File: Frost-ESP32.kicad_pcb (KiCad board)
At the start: 4 copper layers, 50 x 50 mm, 31 parts, among them J1 Micro_SD_Card, J2 CAN, J3 USB_C_Receptacle_USB2.0, J4 Conn_01x10, SW1 SW_Push, U1 ESP32-C3-WROOM-02, U2 AP2112K-3.3, U3 TJA1051T-3

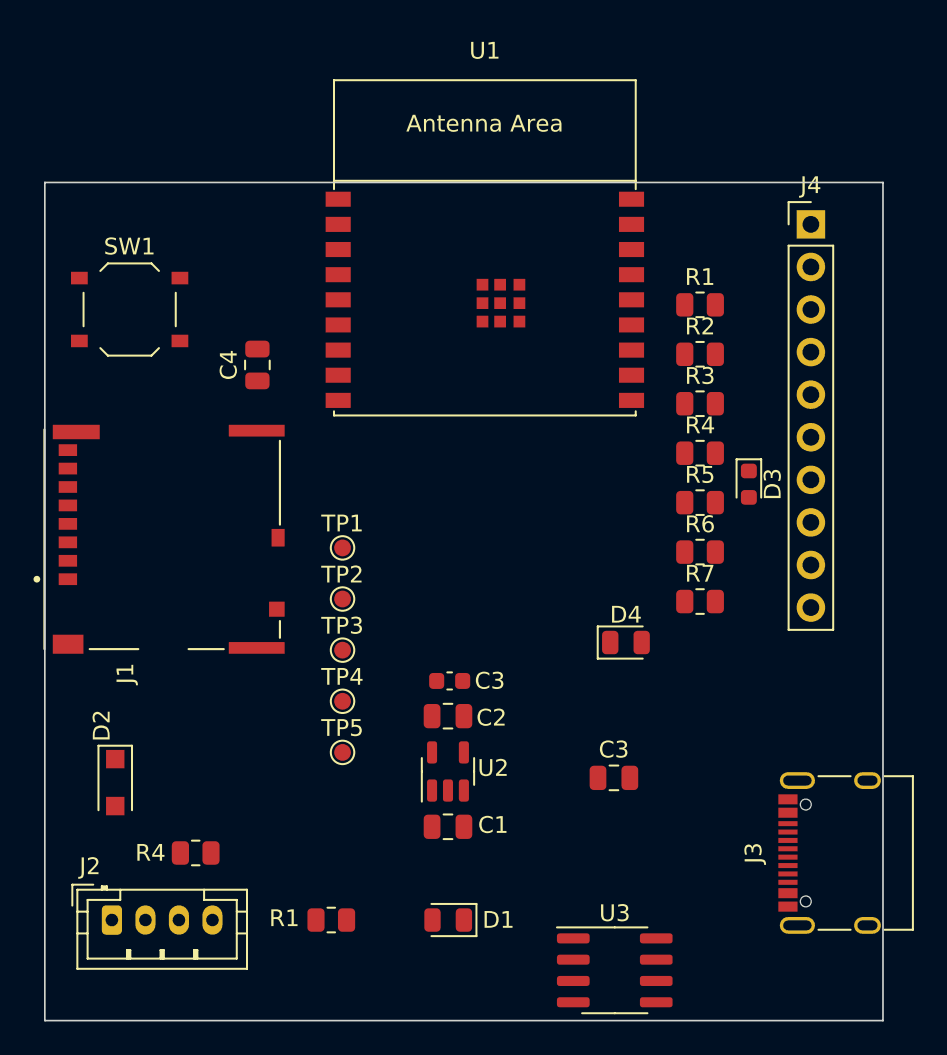
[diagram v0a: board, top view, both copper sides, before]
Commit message: After ordering v0.1
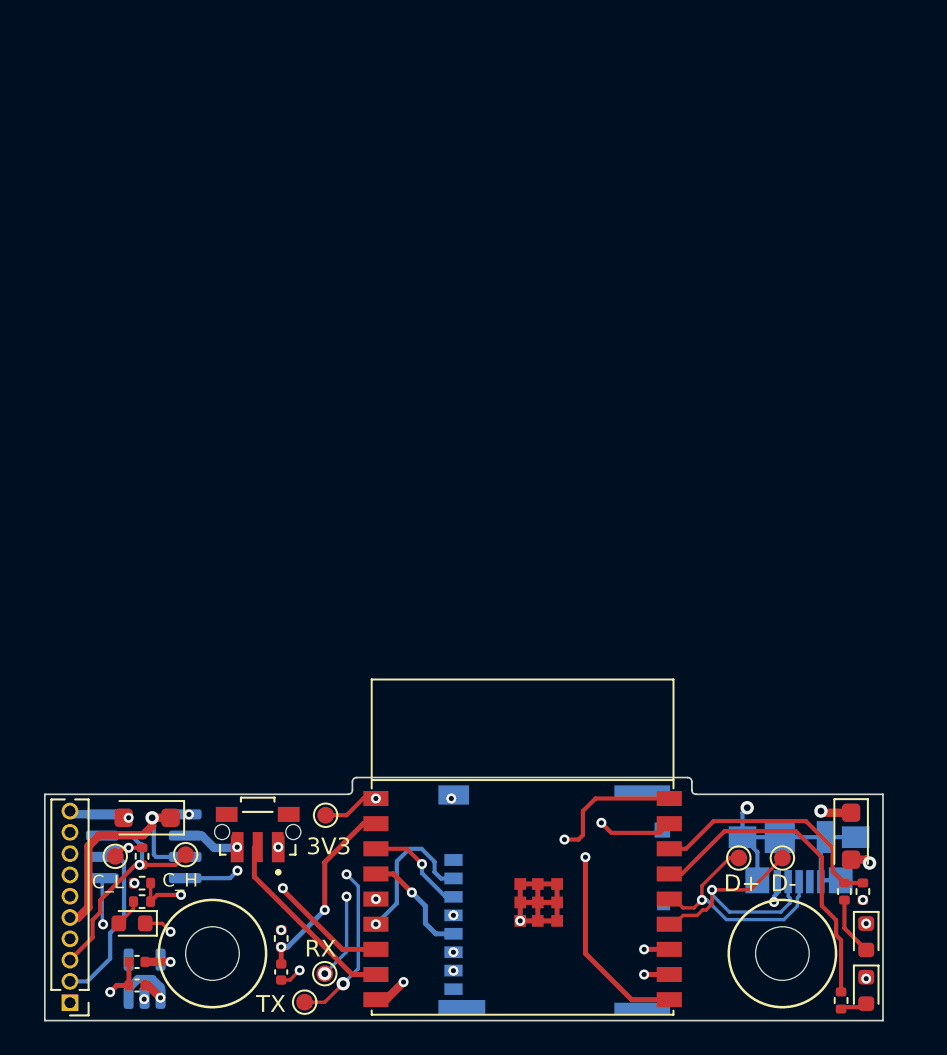
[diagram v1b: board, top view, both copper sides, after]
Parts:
- removed the C3 at (118.2, 90.7)
- removed the C3 at (128.0, 96.5)
- removed C4: 1u, Capacitor_SMD:C_0805_2012Metric
- removed J4: Conn_01x10, Connector_PinHeader_2.54mm:PinHeader_1x10_P2.54mm_Vertical
- removed the R1 at (133.1, 68.3)
- removed the R1 at (111.1, 105.0)
- removed the R4 at (133.1, 77.2)
- removed the R4 at (103.0, 101.0)
- removed SW1: SW_Push, Button_Switch_SMD:SW_Push_1P1T_XKB_TS-1187A
- added C3: 1uF/25V, Capacitor_SMD:C_0402_1005Metric, F.Cu at (108.1, 108.1)
- added D5: 100V/3A, Diode_SMD:D_SOD-123F, F.Cu at (142.1, 100.0)
- added H1: MountingHole, MountingHole:MountingHole_3.2mm_M3, F.Cu at (104.0, 107.0)
- added H2: MountingHole, MountingHole:MountingHole_3.2mm_M3, F.Cu at (138.0, 107.0)
- added R1: 1k, Resistor_SMD:R_0402_1005Metric, F.Cu at (141.7, 103.3)
- added R4: 220, Resistor_SMD:R_0402_1005Metric, F.Cu at (99.8, 101.2)
- added S1: TL3340AF160QG, Fair:SW_TL3340AF160QG, F.Cu at (106.7, 99.8)
- added TP6: TestPoint, TestPoint:TestPoint_Pad_D1.0mm, F.Cu at (110.7, 108.2)
- added TP7: TestPoint, TestPoint:TestPoint_Pad_D1.0mm, F.Cu at (109.5, 109.9)
- C1, C2: value 10uF -> 10uF/6.3V; footprint Capacitor_SMD:C_0805_2012Metric -> Capacitor_SMD:C_0402_1005Metric
- D1: value RED -> Red; footprint LED_SMD:LED_0805_2012Metric -> LED_SMD:LED_0603_1608Metric
- D3: value BLUE -> Blue
- D4: value RED -> Emerald; footprint LED_SMD:LED_0805_2012Metric -> LED_SMD:LED_0603_1608Metric
- J1: footprint espressif:MOLEX_503398-1892 -> Fair:MOLEX_503398-1892; moved to B.Cu
- J2: footprint Connector_JST:JST_PH_B4B-PH-K_1x04_P2.00mm_Vertical -> Connector_PinHeader_1.27mm:PinHeader_1x10_P1.27mm_Vertical
- J3: value USB_C_Receptacle_USB2.0 -> USB__B_Micro_Horizontal; footprint Connector_USB:USB_C_Receptacle_XKB_U262-16XN-4BVC11 -> Connector_USB:USB_Micro-B_Molex_47346-0001; moved to B.Cu
- R2: value R_0805_10k -> 10k; footprint Resistor_SMD:R_0805_2012Metric -> Resistor_SMD:R_0402_1005Metric
- R3, R5, R6, R7: footprint Resistor_SMD:R_0805_2012Metric -> Resistor_SMD:R_0402_1005Metric
- U2, U3: moved to B.Cu
- moved R2 42.9 mm to (108.1, 106.1), turned to 90 degrees
- moved R6 38.7 mm to (99.8, 102.8), turned to 180 degrees
- moved R7 37.8 mm to (99.8, 103.9), turned to 180 degrees
- moved U1 35.8 mm to (122.5, 103.7)
- moved J1 31.5 mm to (124.0, 103.8), turned to -90 degrees
- moved D3 31.0 mm to (143.0, 109.2)
- moved R5 30.9 mm to (141.5, 109.8), turned to 90 degrees
- moved R3 30.7 mm to (142.8, 103.3), turned to 90 degrees
- moved TP2 30.5 mm to (138.0, 101.3)
- moved U3 29.1 mm to (99.9, 100.6), turned to 180 degrees
- moved TP3 26.7 mm to (135.4, 101.3)
- moved C2 23.6 mm to (99.5, 107.5), turned to 180 degrees
- moved D4 22.7 mm to (143.0, 106.0), turned to -90 degrees
- moved U2 21.9 mm to (100.0, 108.5)
- moved C1 20.8 mm to (99.5, 108.9), turned to 180 degrees
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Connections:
- net Net-(D2-A) renamed /Vconn
- R2 pad 1: +3V3 -> Net-(U1-EN/CHIP_PU)
- R2 pad 2: Net-(U1-EN/CHIP_PU) -> +3V3
- R3 pad 2: /LED_RED -> /LED_Green
- R5 pad 1: Net-(D4-A) -> Net-(D3-A)
- R5 pad 2: /LED_RED -> /LED_Blue
- R6 pad 1: /GPIO8 -> +3V3
- R6 pad 2: +3V3 -> /GPIO8
- R7 pad 1: Net-(D3-A) -> +3V3
- R7 pad 2: /LED_BLUE -> Net-(D1-A)
- U1 pad 15: /LED_BLUE -> /LED_Blue
- U1 pad 16: /LED_RED -> /LED_Green
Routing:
- net +5V: track 0.00 -> 78.4 mm, vias 0 -> 3
- net /TX: track 0.00 -> 49.0 mm, vias 0 -> 3
- net /RX: track 0.00 -> 44.9 mm, vias 0 -> 3
- net /GPIO10: track 0.00 -> 44.7 mm, vias 0 -> 1
- net GND: track 0.00 -> 44.3 mm, vias 0 -> 13
- net /CAN_RX: track 0.00 -> 31.8 mm, vias 0 -> 2
- net /CAN_TX: track 0.00 -> 29.6 mm, vias 0 -> 2
- net /GPIO8: track 0.00 -> 20.8 mm, vias 0 -> 2
- net /LED_Blue: track 0.00 -> 19.3 mm
- net /USB_D-: track 0.00 -> 15.3 mm, vias 0 -> 1
- net /LED_Green: track 0.00 -> 14.6 mm
- net /CANH: track 0.00 -> 14.3 mm, vias 0 -> 1
- net /CANL: track 0.00 -> 14.1 mm, vias 0 -> 1
- net /USB_D+: track 0.00 -> 13.7 mm, vias 0 -> 1
- net /Vconn: track 0.00 -> 12.8 mm, vias 0 -> 1
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- added copper zone on In2.Cu, net +3V3
- added copper zone on In1.Cu, net GND
- added copper zone on In4.Cu, net GND
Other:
- board size 50 x 50 mm -> 50 x 14.5 mm
- copper layers 4 -> 6
- board text added: "3V3"
- board text added: "5V In"
- board text added: "5V Out"
- board text added: "CANH"
- board text added: "CANL"
- board text added: "C_H"
- board text added: "C_L"
- board text added: "D+"
- board text added: "D-"
- board text added: "GND"
- board text added: "IO08"
- board text added: "IO10"
- board text added: "RX"
- board text added: "TX"
